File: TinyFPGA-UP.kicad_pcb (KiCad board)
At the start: 2 copper layers, 17.8 x 35.6 mm, 35 parts, among them J1 Conn_01x14, J2 Conn_01x14, J3 USB_B_Micro, J4 Conn_02x08_Odd_Even, J5 Conn_02x03_Odd_Even, SW1 SW_Push, U1 iCE40-UP5K-SG48, U2 MIC5504-3.3, U3 DSC6001CI2A, U4 MIC5365-1.2, U5 AT25SF081

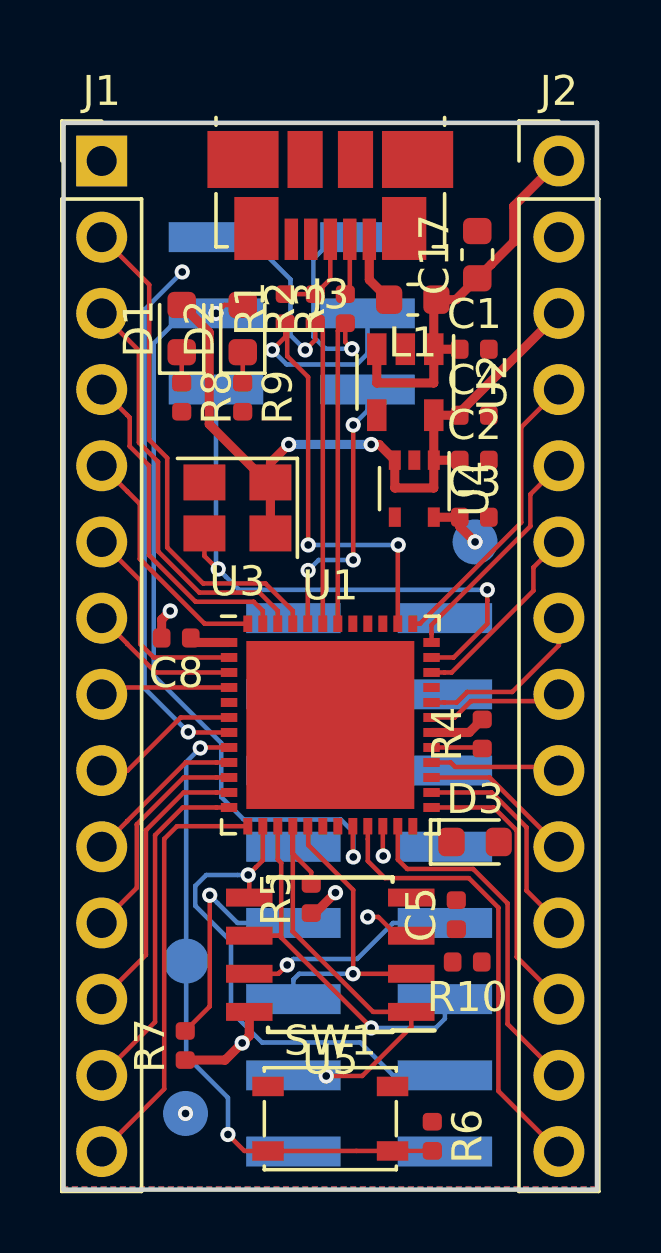
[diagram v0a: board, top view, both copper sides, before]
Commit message: Update routing
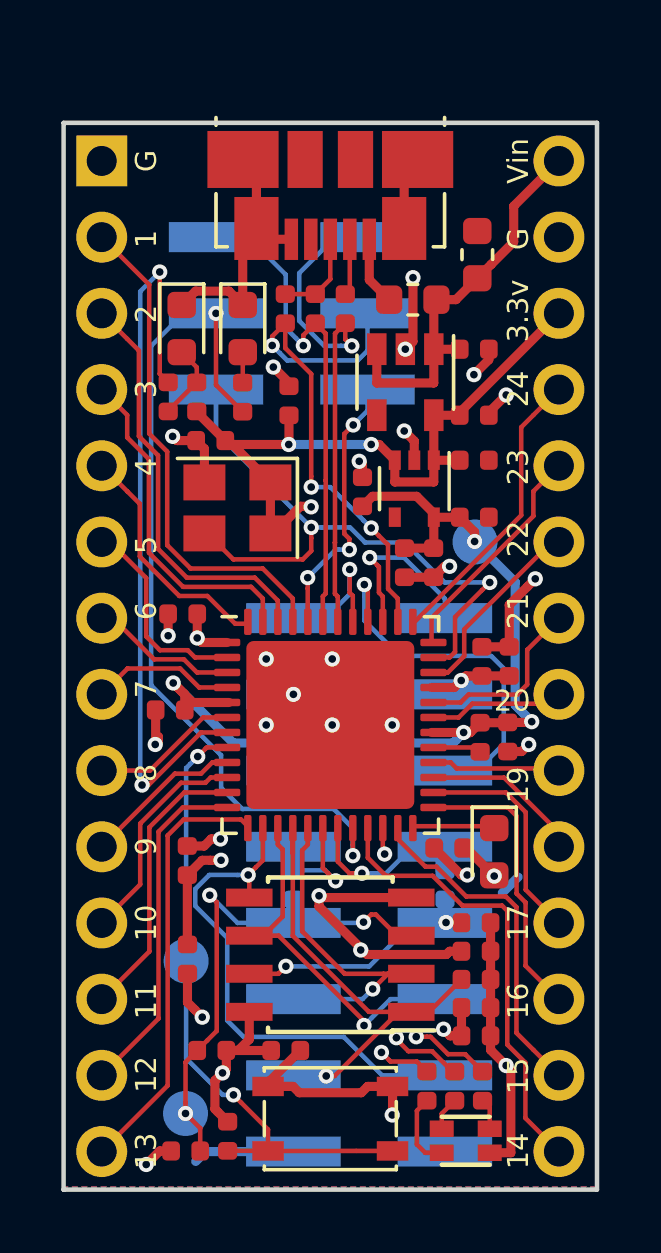
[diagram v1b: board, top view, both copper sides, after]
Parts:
- added C10: 100nF, Capacitor_SMD:C_0402_1005Metric, F.Cu at (145.8, 116.1)
- added C11: 100nF, Capacitor_SMD:C_0402_1005Metric, F.Cu at (156.2, 114.5)
- added C12: 100nF, Capacitor_SMD:C_0402_1005Metric, F.Cu at (156.0, 124.1)
- added C13: 100nF, Capacitor_SMD:C_0402_1005Metric, F.Cu at (146.2, 112.9)
- added C14: 100nF, Capacitor_SMD:C_0402_1005Metric, F.Cu at (153.6, 111.2)
- added C15: 100nF, Capacitor_SMD:C_0402_1005Metric, F.Cu at (157.1, 114.5)
- added C16: 100nF, Capacitor_SMD:C_0402_1005Metric, F.Cu at (146.4, 121.1)
- added C18: 100nF, Capacitor_SMD:C_0402_1005Metric, F.Cu at (146.4, 124.4)
- added C19: 100nF, Capacitor_SMD:C_0402_1005Metric, F.Cu at (152.2, 108.8)
- added C20: 100nF, Capacitor_SMD:C_0402_1005Metric, F.Cu at (149.8, 105.8)
- added C21: 100nF, Capacitor_SMD:C_0402_1005Metric, F.Cu at (156.0, 127.0)
- added C22: 100nF, Capacitor_SMD:C_0402_1005Metric, F.Cu at (156.0, 126.0)
- added C6: 10uF, Capacitor_SMD:C_0402_1005Metric, F.Cu at (157.1, 117.0)
- added C7: 100nF, Capacitor_SMD:C_0402_1005Metric, F.Cu at (155.1, 120.7)
- added C9: 100nF, Capacitor_SMD:C_0402_1005Metric, F.Cu at (154.6, 111.2)
- added D4: RGB, DRA818:LTST-C19HE1WT, F.Cu at (155.7, 130.5)
- added R11: 0, Resistor_SMD:R_0402_1005Metric, F.Cu at (145.7, 105.7)
- added R12: 100, Resistor_SMD:R_0402_1005Metric, F.Cu at (156.2, 128.6)
- added R13: 100, Resistor_SMD:R_0402_1005Metric, F.Cu at (155.3, 128.6)
- added R14: 100, Resistor_SMD:R_0402_1005Metric, F.Cu at (154.4, 128.6)
- added R15: DNP, Resistor_SMD:R_0402_1005Metric, F.Cu at (146.3, 130.8)
- added R16: 0, Resistor_SMD:R_0402_1005Metric, B.Cu at (155.0, 121.9)
- added R17: 0, Resistor_SMD:R_0402_1005Metric, B.Cu at (149.9, 121.9)
- added REF**: OSHW-Logo2_7.3x6mm_SilkScreen, Symbol:OSHW-Logo2_7.3x6mm_SilkScreen, B.Cu at (151.6, 109.4)
- R8: value 270 -> 2.2k
- moved C5 17.8 mm to (147.2, 107.1), turned to 180 degrees
- moved C8 14.2 mm to (149.7, 127.5), turned to 0 degrees
- moved R6 6.82 mm to (147.7, 130.3)
- moved R5 6.12 mm to (156.0, 125.1), turned to 180 degrees
- moved R10 1.34 mm to (156.0, 123.2)
- moved R7 0.90 mm to (147.2, 127.5), turned to 180 degrees
- moved D3 0.72 mm to (156.6, 120.8), turned to 270 degrees
- moved R8 0.50 mm to (146.7, 105.7), turned to 90 degrees
- moved R4 0.13 mm to (156.1, 117.0)
- turned D1 to 270 degrees
- turned D2 to 270 degrees
- turned R9 to 90 degrees
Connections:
- D1 pad 1: Net-(D1-Pad1) -> GND
- D1 pad 2: +3V3 -> Net-(D1-Pad2)
- D2 pad 1: Net-(D2-Pad1) -> GND
- D2 pad 2: LED -> Net-(D2-Pad2)
- J3 pad 4: (no net) -> Net-(J3-Pad4)
- J4 pad 1: (no net) -> RGB0
- J4 pad 2: (no net) -> RGB2
- J4 pad 5: (no net) -> RGB1
- J4 pad 6: (no net) -> Net-(J4-Pad6)
- J4 pad 7: (no net) -> 29B
- J4 pad 8: (no net) -> 31B
- R8 pad 1: Net-(D1-Pad1) -> +3V3
- R8 pad 2: GND -> Net-(D1-Pad2)
- R9 pad 1: Net-(D2-Pad1) -> LED
- R9 pad 2: GND -> Net-(D2-Pad2)
- U1 pad 18: (no net) -> 31B
- U1 pad 19: (no net) -> 29B
- U1 pad 39: (no net) -> RGB0
- U1 pad 40: (no net) -> RGB1
- U1 pad 41: (no net) -> RGB2
- U1 pad 7: (no net) -> CDONE
- U2 pad 4: (no net) -> Net-(U2-Pad4)
- U4 pad 4: (no net) -> Net-(U4-Pad4)
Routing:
- net GND: track 1.65 -> 57.2 mm, vias 1 -> 27
- net RGB1: track 0.00 -> 32.5 mm, vias 0 -> 2
- net +1V2: track 3.77 -> 30.8 mm, vias 1 -> 4
- net RGB0: track 0.00 -> 25.8 mm, vias 0 -> 2
- net CDONE: track 0.00 -> 24.8 mm, vias 0 -> 2
- net RGB2: track 0.00 -> 24.1 mm, vias 0 -> 2
- net +3V3: track 32.0 -> 50.9 mm, vias 5 -> 10
- net (no net): track 17.8 -> 0.00 mm, vias 2 -> 0
- net WP: track 9.84 -> 17.6 mm
- net 29B: track 0.00 -> 6.06 mm, vias 0 -> 1
- net 31B: track 0.00 -> 4.33 mm, vias 0 -> 1
- net Net-(D3-Pad1): track 0.00 -> 2.75 mm
- net Net-(D1-Pad2): track 0.00 -> 2.58 mm
- net Net-(D4-Pad1): track 0.00 -> 2.54 mm
- net LED: track 27.4 -> 29.9 mm
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- added copper zone on In2.Cu, net +3V3
- added copper zone on In1.Cu, net GND
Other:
- copper layers 2 -> 4
- board text added: "1"
- board text added: "1.2v"
- board text added: "10"
- board text added: "11"
- board text added: "12"
- board text added: "13"
- board text added: "14"
- board text added: "15"
- board text added: "16"
- board text added: "17"
- board text added: "18"
- board text added: "19"
- board text added: "2"
- board text added: "20"
- board text added: "21"
- board text added: "22"
- board text added: "23"
- board text added: "24"
- board text added: "27"
- board text added: "28"
- board text added: "3"
- board text added: "3.3v"
- board text added: "31"
- board text added: "4"
- board text added: "5"
- board text added: "6"
- board text added: "7"
- board text added: "8"
- board text added: "9"
- board text added: "CLK"
- board text added: "DinyFPGA UP"
- board text added: "G"
- board text added: "GND"
- board text added: "HB9GPC"
- board text added: "HLD"
- board text added: "LD0"
- board text added: "LD1"
- board text added: "LD2"
- board text added: "LED"
- board text added: "NC"
- board text added: "PU"
- board text added: "RST"
- board text added: "SCK"
- board text added: "SDI"
- board text added: "SDO"
- board text added: "SS"
- board text added: "U+"
- board text added: "U-"
- board text added: "Vin"
- board text added: "WP"
- board text added: "rev. A"
